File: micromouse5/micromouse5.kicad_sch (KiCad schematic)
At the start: 71 parts, among them J1 Conn_01x06_Pin, J2 Conn_01x06_Pin, J3 JST 2, J4 JST 1, J5 Conn_01x04_Pin, Q1 IR Receiver, Q2 IR Receiver, Q3 IR Receiver, Q4 IR Receiver, SW1 Button, SW2 EG1218, U1 HBridge, U2 Voltage Regulator, U3 MOSFET, U4 MOSFET, U5 MOSFET, U6 MOSFET, U7 STM32F205RGTx

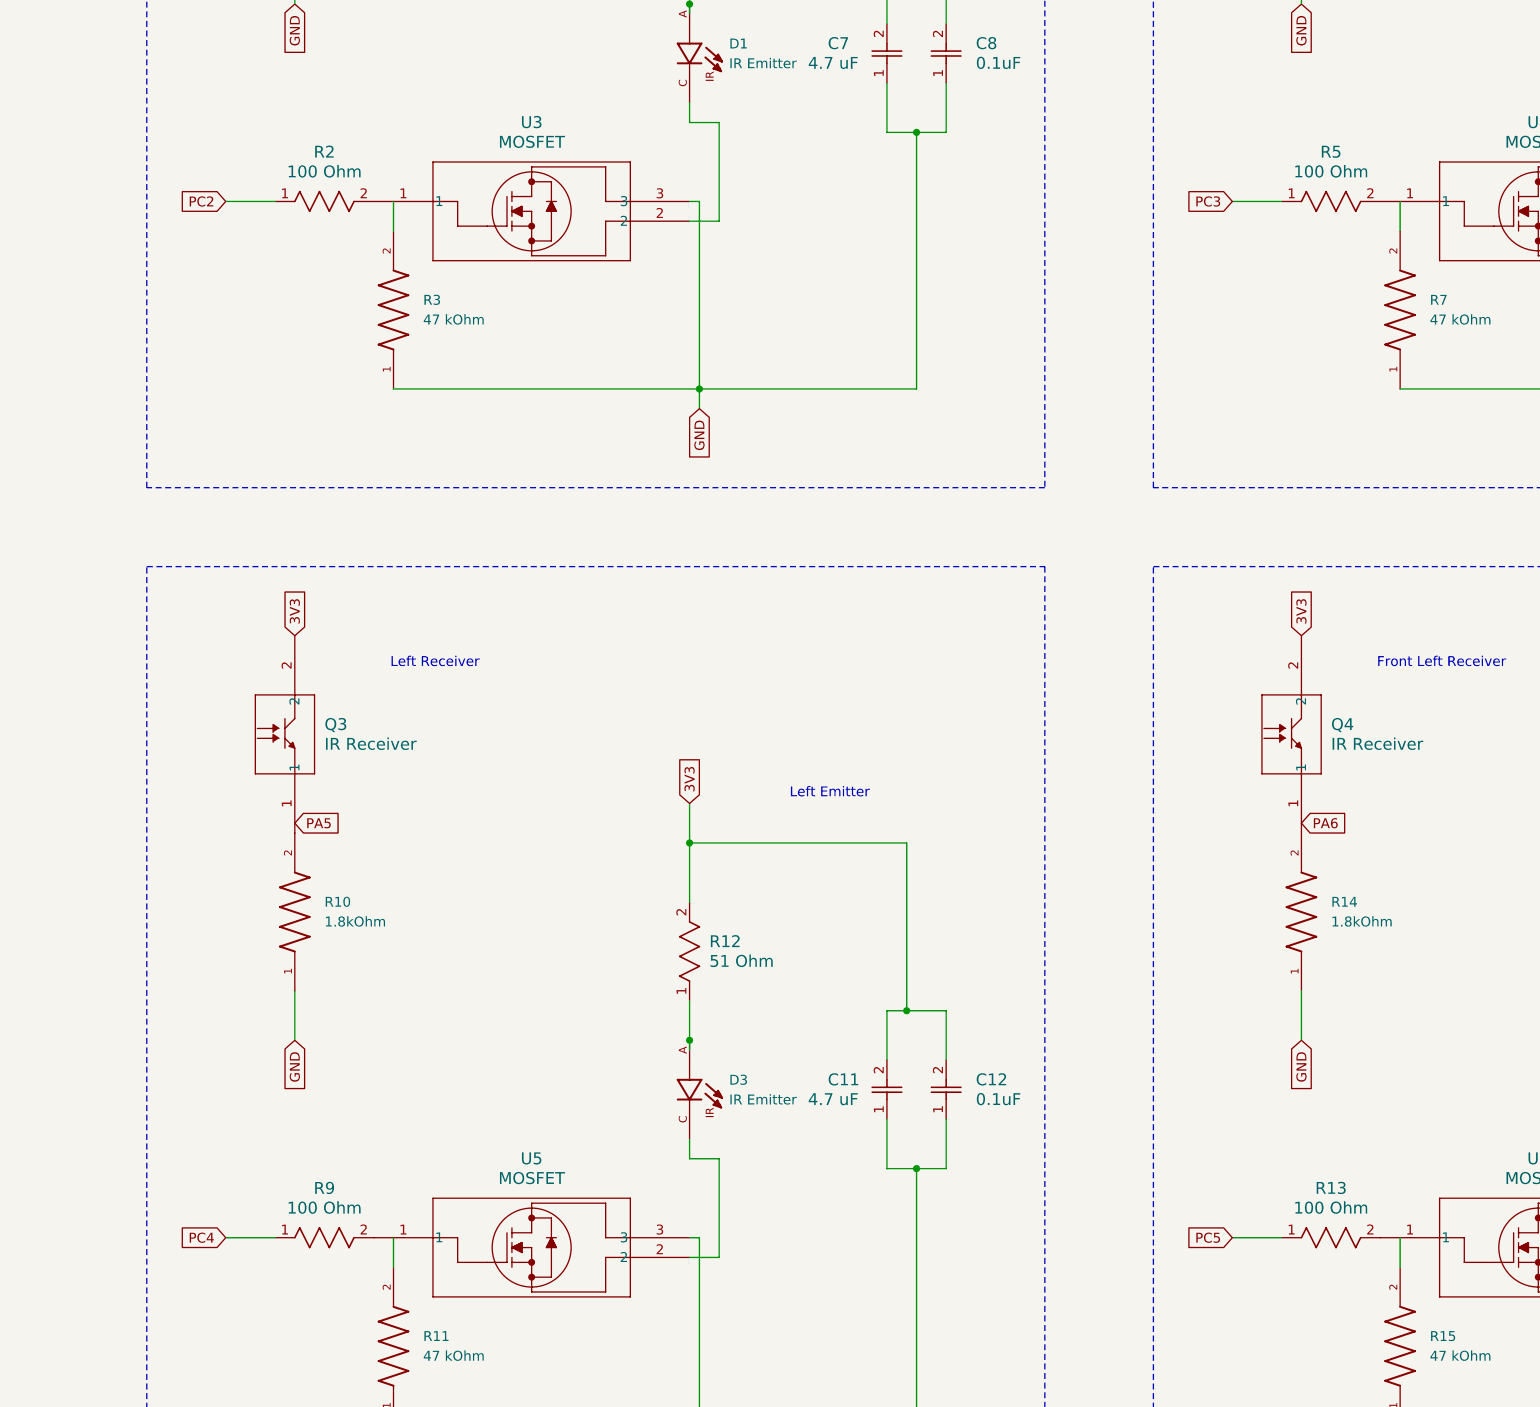
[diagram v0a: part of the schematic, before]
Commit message: PCB work
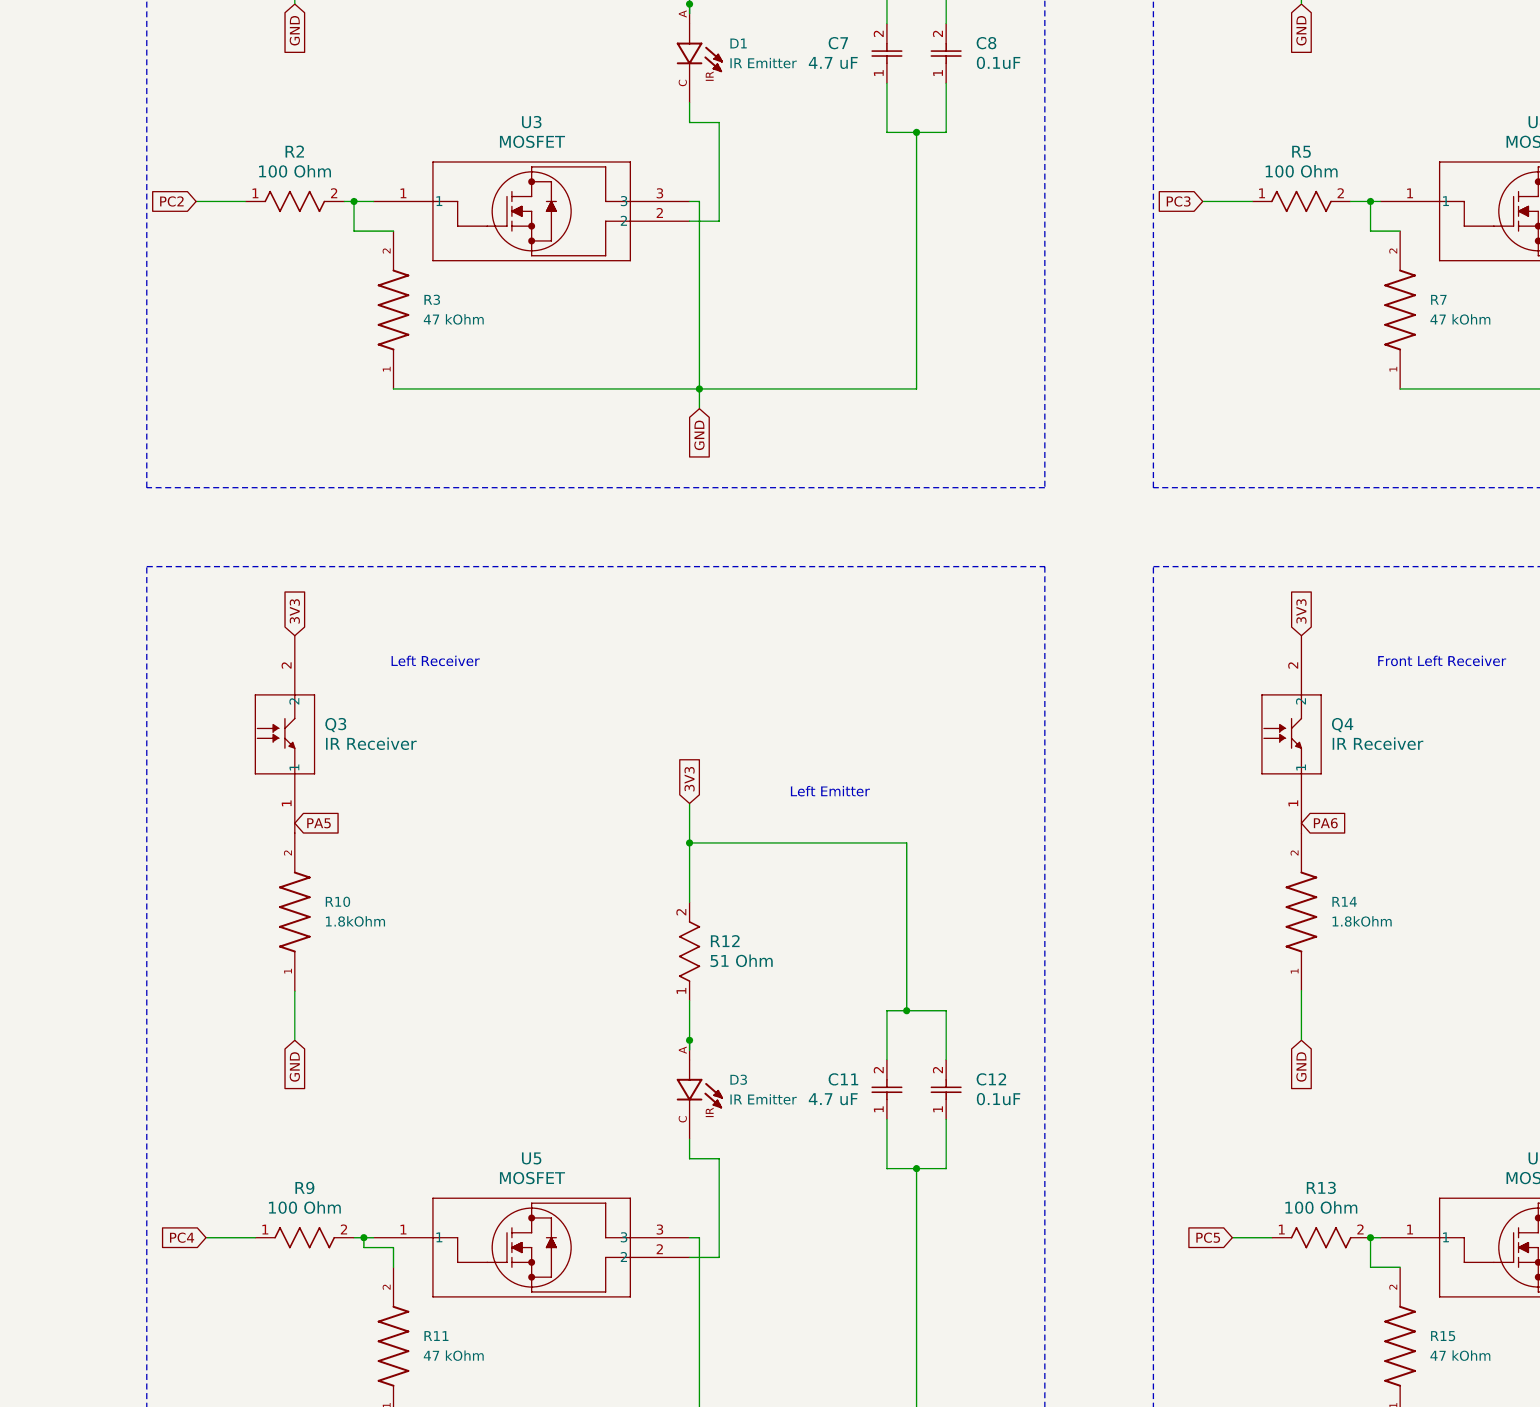
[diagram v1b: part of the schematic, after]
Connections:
- net at R2.2, U3.1: now also R3.2
- net at R5.2, U4.1: now also R7.2
- net at R15.2: now also R13.2, U6.1
- net at R11.2: now also R9.2, U5.1
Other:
- moved on the sheet: R13, R2, R5, R9
